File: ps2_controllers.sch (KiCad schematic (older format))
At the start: 11 parts

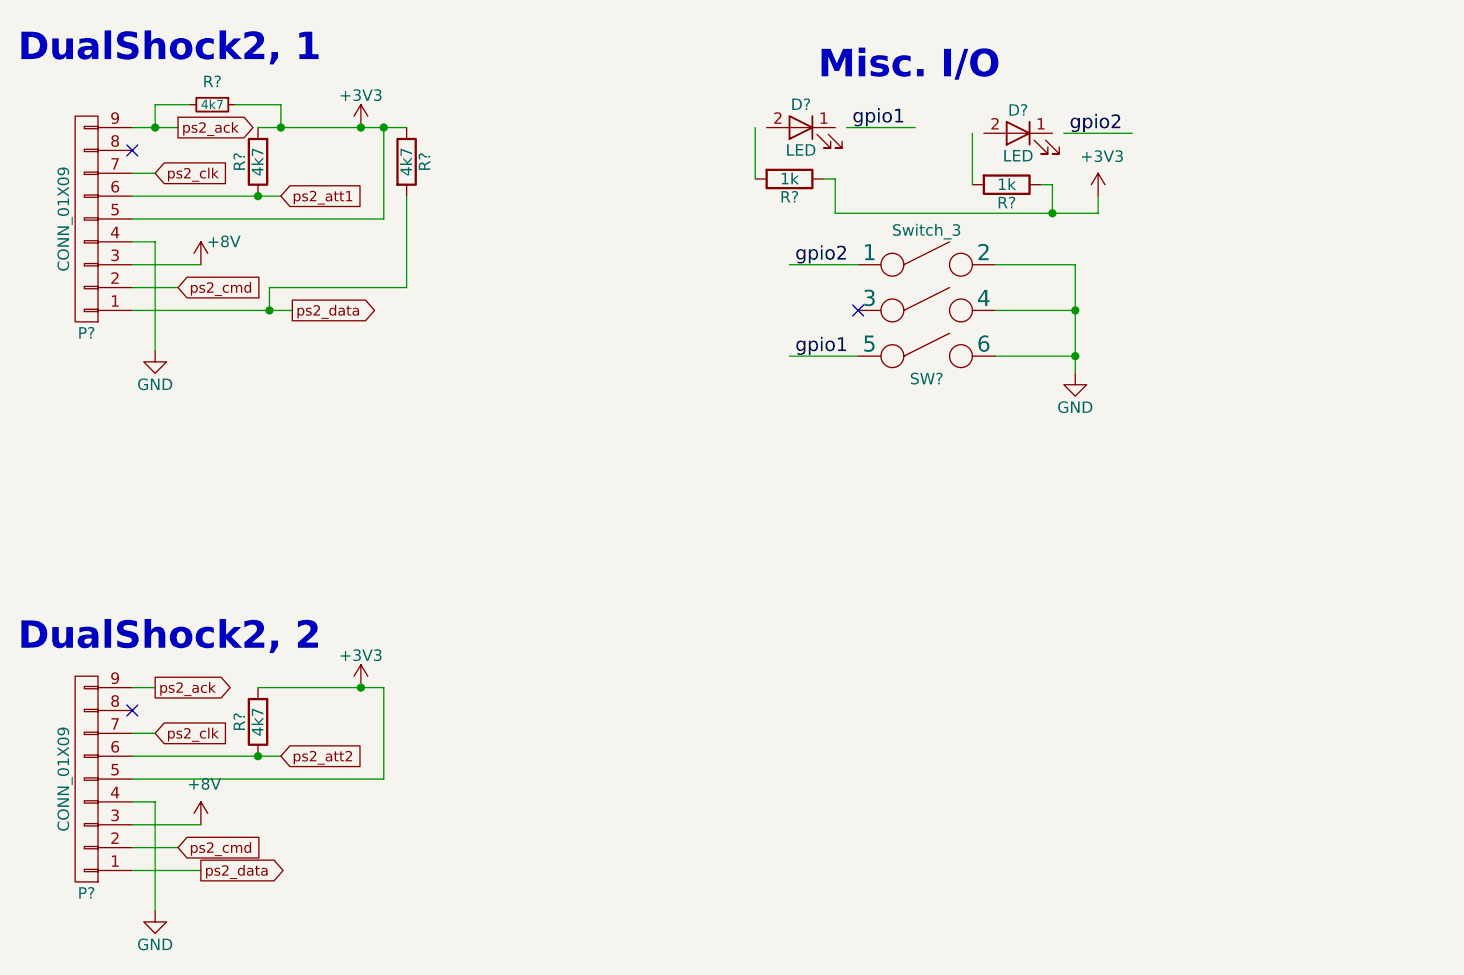
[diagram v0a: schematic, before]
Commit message: Passing ERC
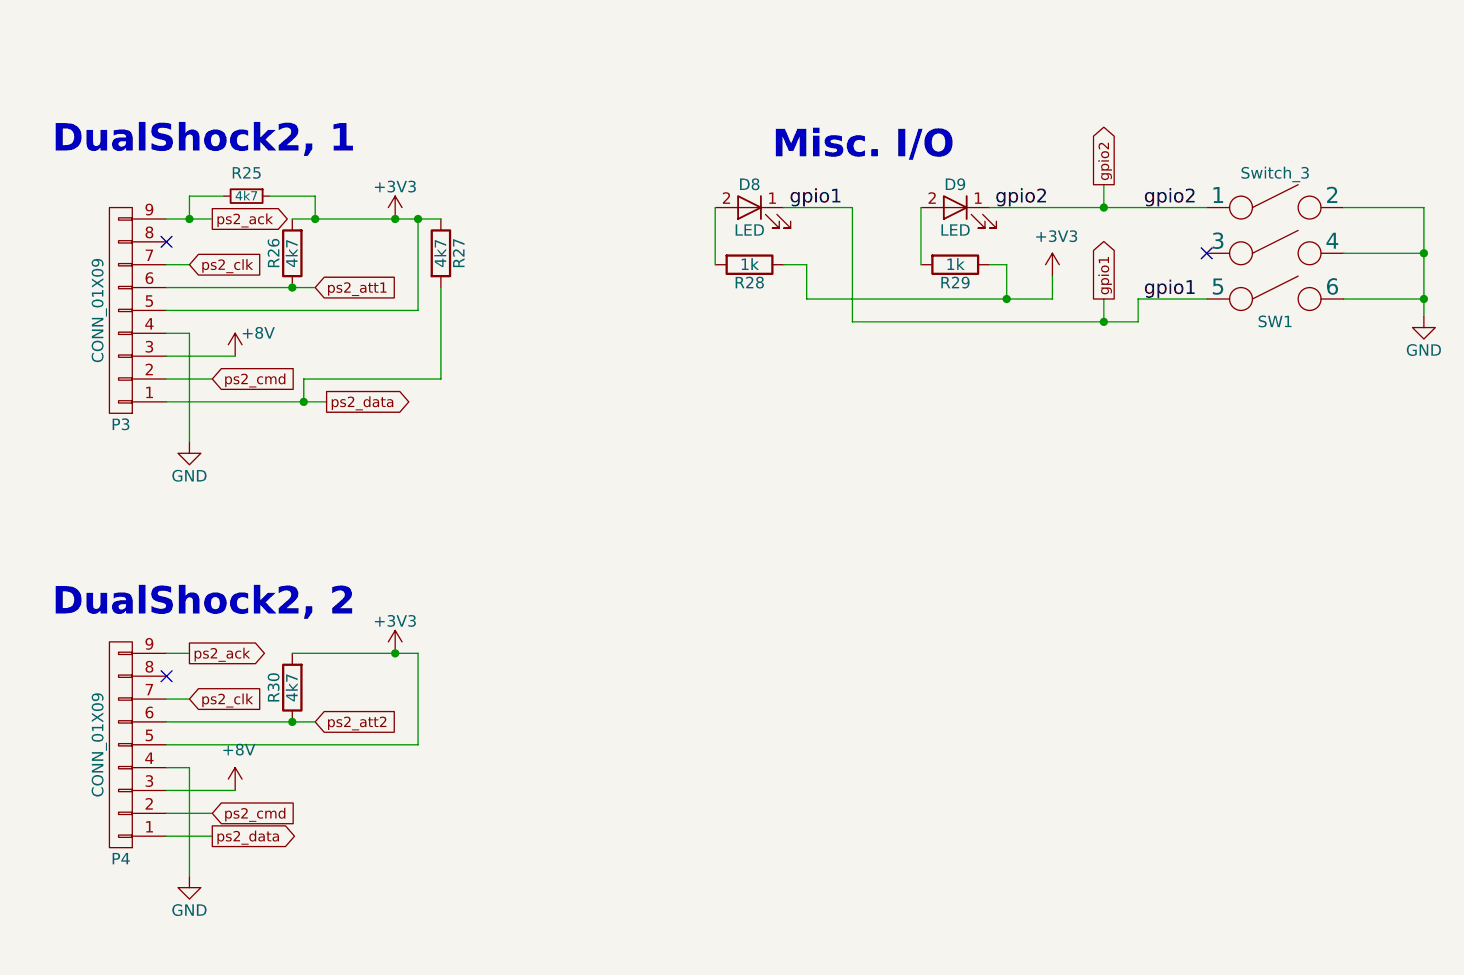
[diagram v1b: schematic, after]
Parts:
- gave numbers to parts that had none: 11
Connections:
- wire segments 45 -> 49
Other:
- moved on the sheet: D8, D9, P3, P4, R25, R26, R27, R28, R29, R30, SW1

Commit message: Starting on netlist
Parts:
- R25: footprint (none) -> Resistors_SMD:R_0603
- R26, R27, R30: footprint Resistors_SMD:R_0805_HandSoldering -> Resistors_SMD:R_0603
- R28, R29: footprint Resistors_SMD:R_0805_HandSoldering -> Resistors_SMD:R_0805
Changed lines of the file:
@@
 LIBS:w_device
 LIBS:pcb_ledtorus_controller-cache
-LIBS:tiva_pcb1-cache
 EELAYER 26 0
 EELAYER END
@@
 F 0 "R28" V 4130 1800 50  0000 C CNN
 F 1 "1k" V 4050 1800 50  0000 C CNN
-F 2 "Resistors_SMD:R_0805_HandSoldering" V 3980 1800 30  0001 C CNN
+F 2 "Resistors_SMD:R_0805" V 3980 1800 30  0001 C CNN
 F 3 "" H 4050 1800 30  0000 C CNN
 	1    4050 1800
@@
 F 0 "R29" V 5030 1800 50  0000 C CNN
 F 1 "1k" V 4950 1800 50  0000 C CNN
-F 2 "Resistors_SMD:R_0805_HandSoldering" V 4880 1800 30  0001 C CNN
+F 2 "Resistors_SMD:R_0805" V 4880 1800 30  0001 C CNN
 F 3 "" H 4950 1800 30  0000 C CNN
 	1    4950 1800
@@
 F 0 "R26" V 2130 1750 50  0000 C CNN
 F 1 "4k7" V 2050 1750 50  0000 C CNN
-F 2 "Resistors_SMD:R_0805_HandSoldering" V 1980 1750 30  0001 C CNN
+F 2 "Resistors_SMD:R_0603" V 1980 1750 30  0001 C CNN
 F 3 "" H 2050 1750 30  0000 C CNN
 	1    2050 1750
@@
 F 0 "R30" V 2130 3650 50  0000 C CNN
 F 1 "4k7" V 2050 3650 50  0000 C CNN
-F 2 "Resistors_SMD:R_0805_HandSoldering" V 1980 3650 30  0001 C CNN
+F 2 "Resistors_SMD:R_0603" V 1980 3650 30  0001 C CNN
 F 3 "" H 2050 3650 30  0000 C CNN
 	1    2050 3650
@@
 F 0 "R27" V 2780 1750 50  0000 C CNN
 F 1 "4k7" V 2700 1750 50  0000 C CNN
-F 2 "Resistors_SMD:R_0805_HandSoldering" V 2630 1750 30  0001 C CNN
+F 2 "Resistors_SMD:R_0603" V 2630 1750 30  0001 C CNN
 F 3 "" H 2700 1750 30  0000 C CNN
 	1    2700 1750
@@
 F 0 "R25" V 1750 1500 50  0000 C CNN
 F 1 "4k7" V 1850 1500 40  0000 C CNN
-F 2 "" H 1850 1500 50  0001 C CNN
+F 2 "Resistors_SMD:R_0603" H 1850 1500 50  0001 C CNN
 F 3 "" H 1850 1500 50  0001 C CNN
 	1    1850 1500
